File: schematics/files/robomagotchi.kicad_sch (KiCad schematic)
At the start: 24 parts, among them M1 Servo Motor, U1 SPI TFT Display (ST7735), U2 I2C OLED Display (SSD1306), U3 Ultrasonic Proximity Sensor (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, U4 Temp Sensor (DHT11), U5 IR Receiver (VS18838B)

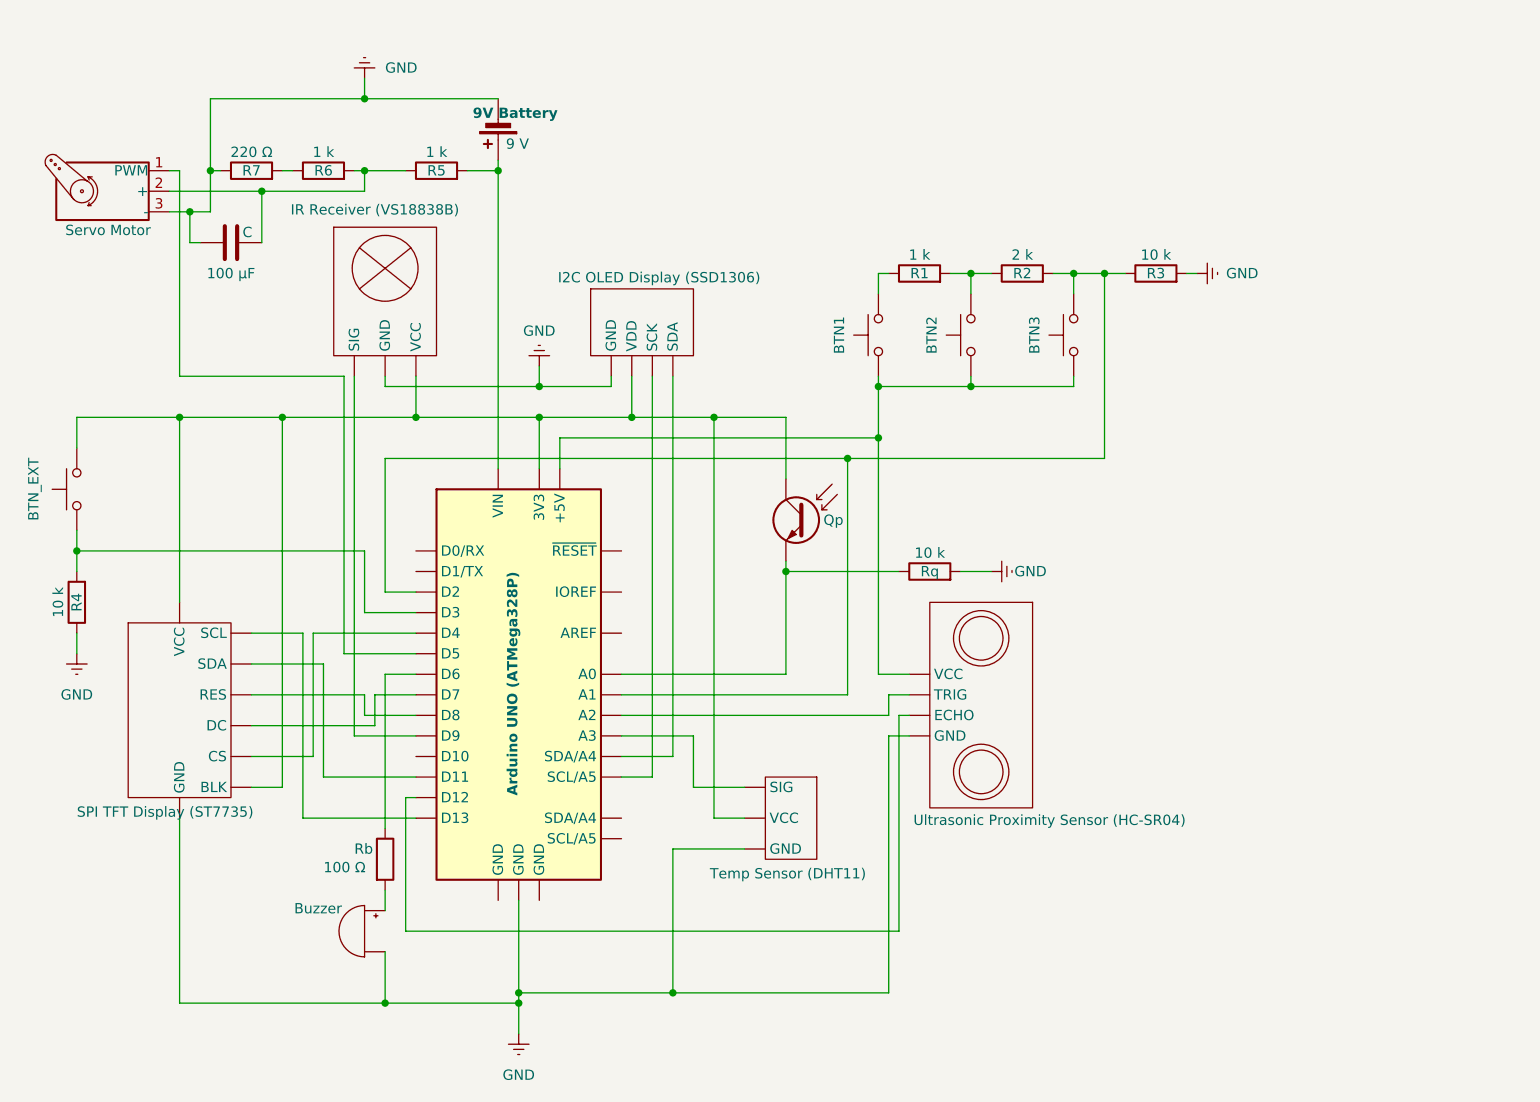
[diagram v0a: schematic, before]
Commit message: Updated README, BoM and Schematic
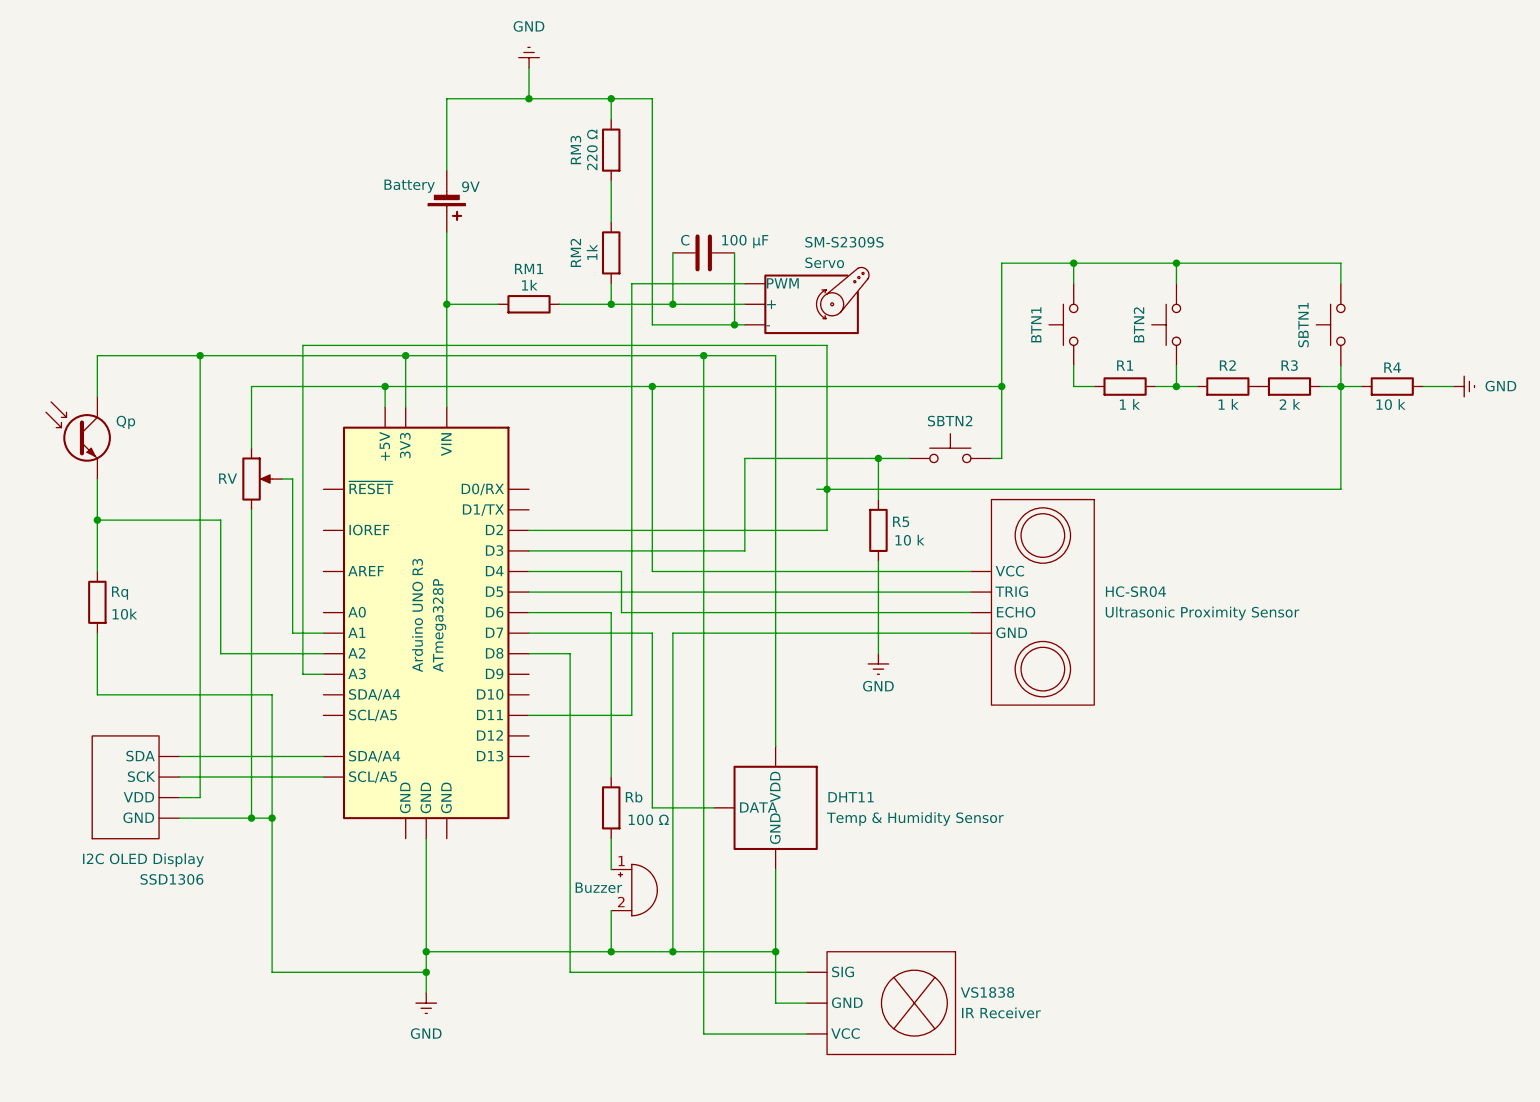
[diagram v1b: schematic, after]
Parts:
- removed A2: Arduino UNO (ATMega328P), Module:Arduino_UNO_R3, symbol MCU_Module:Arduino_UNO_R3
- removed BT2: 9 V, symbol Device:Battery_Cell
- removed BTN2, BTN3, BTN_EXT: SW_Push, symbol Switch:SW_Push
- removed M1: Servo Motor, symbol Motor:Motor_Servo
- removed Qp: Phototransistor, LED_THT:LED_D3.0mm_Clear, symbol Sensor_Optical:SFH309
- removed R6: 1 k, symbol Device:R
- removed R7: 220 Ω, symbol Device:R
- removed U1: SPI TFT Display (ST7735), symbol A_LAPTOP_LIB:ST7735_SPI_TFT_Display
- removed U2: I2C OLED Display (SSD1306), symbol My_Symbols:DISPLAY_096_GM009605_OLED
- removed U3: Ultrasonic Proximity Sensor (HC-SR04), symbol My_Symbols:HCSR04_PROXIMITY_SENSOR
- removed U4: Temp Sensor (DHT11), symbol My_Symbols:TMP36_TEMPERATURE_SENSOR
- removed U5: IR Receiver (VS18838B), symbol My_Symbols:VS1838B_IR_RECEIVER
- added ATmega328P: Arduino UNO R3, Module:Arduino_UNO_R3, symbol MCU_Module:Arduino_UNO_R3
- added Battery: 9V, symbol Device:Battery_Cell
- added DHT11: Temp & Humidity Sensor, Sensor:Aosong_DHT11_5.5x12.0_P2.54mm, symbol Sensor:DHT11
- added HC-SR04: Ultrasonic Proximity Sensor, symbol My_Symbols:HCSR04_PROXIMITY_SENSOR
- added Qp: Phototransistor, LED_THT:LED_D5.0mm_Clear, symbol Sensor_Optical:BPW40
- added RM1, RM2: 1k, symbol Device:R
- added RM3: 220 Ω, symbol Device:R
- added RV: R_Potentiometer, symbol Device:R_Potentiometer
- added SBTN1, SBTN2: SW_Push, symbol Switch:SW_Push
- added SBTN_A: BTN2, symbol Switch:SW_Push
- added SM-S2309S: Servo, symbol Motor:Motor_Servo
- added SSD1306: I2C OLED Display, symbol My_Symbols:DISPLAY_096_GM009605_OLED
- added VS1838: IR Receiver, symbol My_Symbols:VS1838B_IR_RECEIVER
- C: value 100 µF -> 100 μF
- R2: value 2 k -> 1 k
- R3: value 10 k -> 2 k
- R5: value 1 k -> 10 k
- Rq: value 10 k -> 10k
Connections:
- net GND: now also R5.1, ATmega328P.6 (GND), Battery.2 (-), DHT11.4 (GND), HC-SR04. (VCC), RM3.1, RV.3, SM-S2309S.3 (-), SSD1306. (VDD), VS1838. (VCC); no longer R3.2
- net at BTN1.2: now also ATmega328P.5 (+5V), HC-SR04. (VCC), RV.1, SBTN1.2, SBTN2.2, SBTN_A.2; no longer R1.1
- net at R2.1: now also R3.2; no longer R1.2
- net at C.2: now also RM1.1, RM2.2, SM-S2309S.2 (+); no longer R5.1
- net at R4.2: now also R3.1, ATmega328P.12 (A3), ATmega328P.17 (D2), SBTN1.1
- net at BTN1.1: now also R1.2
- net at R5.2: now also ATmega328P.18 (D3), SBTN2.1
- net at R2.2: now also R1.1, SBTN_A.1; no longer R3.1
- net at Rb.1: now also ATmega328P.21 (D6)
- net at Rq.1: now also ATmega328P.11 (A2), Qp.2 (E)
- new net: ATmega328P.4 (3V3), DHT11.1 (VDD), Qp.1 (C), SSD1306. (VDD), VS1838. (VCC)
- new net: ATmega328P.10 (A1), RV.2
- new net: ATmega328P.19 (D4), HC-SR04. (VCC)
- new net: ATmega328P.20 (D5), HC-SR04. (VCC)
- new net: ATmega328P.22 (D7), DHT11.2 (DATA)
- new net: ATmega328P.23 (D8), VS1838. (VCC)
- new net: ATmega328P.26 (D11), SM-S2309S.1 (PWM)
- new net: ATmega328P.31 (SDA/A4), SSD1306. (VDD)
- new net: ATmega328P.32 (SCL/A5), SSD1306. (VDD)
- new net: ATmega328P.8 (VIN), Battery.1 (+), RM1.2
- new net: RM2.1, RM3.2
